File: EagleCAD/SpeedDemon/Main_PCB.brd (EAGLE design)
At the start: 77 x 46.5 mm, 77 parts, among them Q1 DMC2700, Q2 BSS138L, U2 NC7S08M, U3 LM3676, U4 STM32F072-LQFP48, X1 32.768kHz

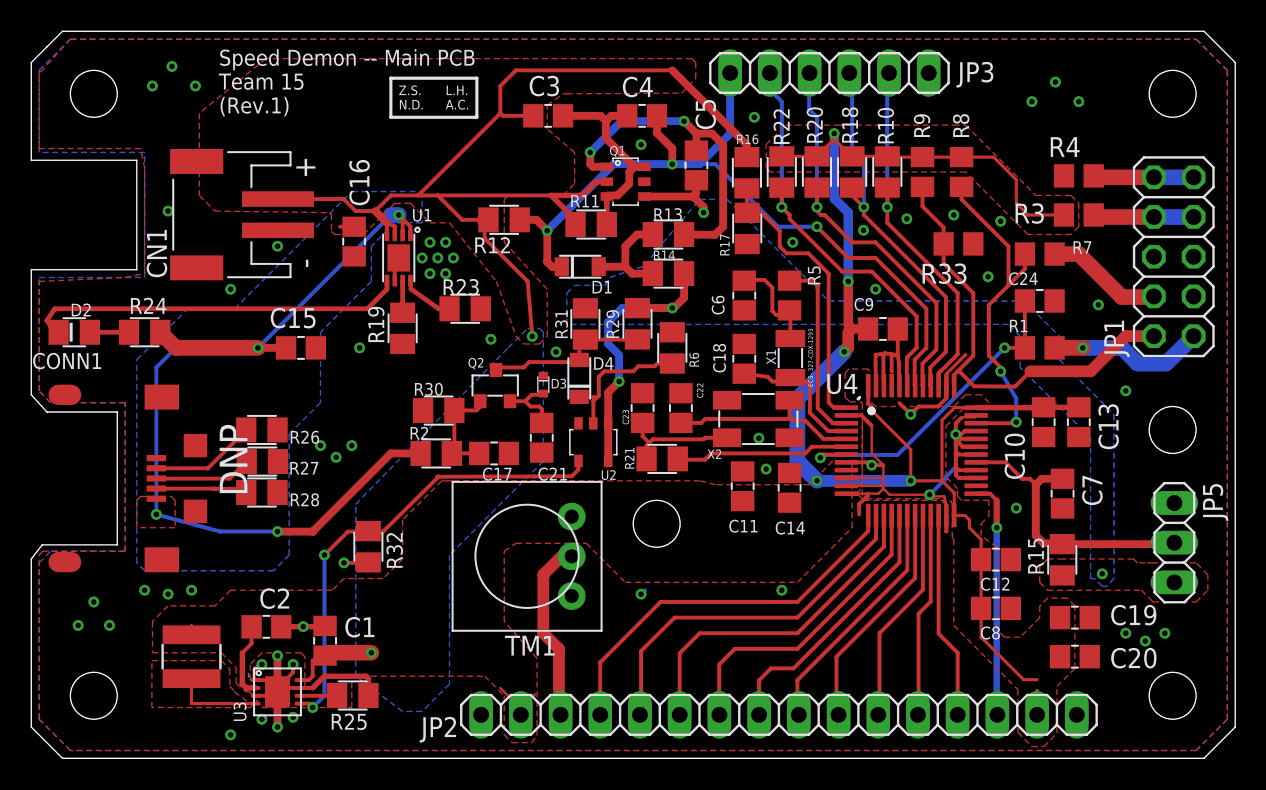
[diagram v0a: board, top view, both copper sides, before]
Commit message: final board
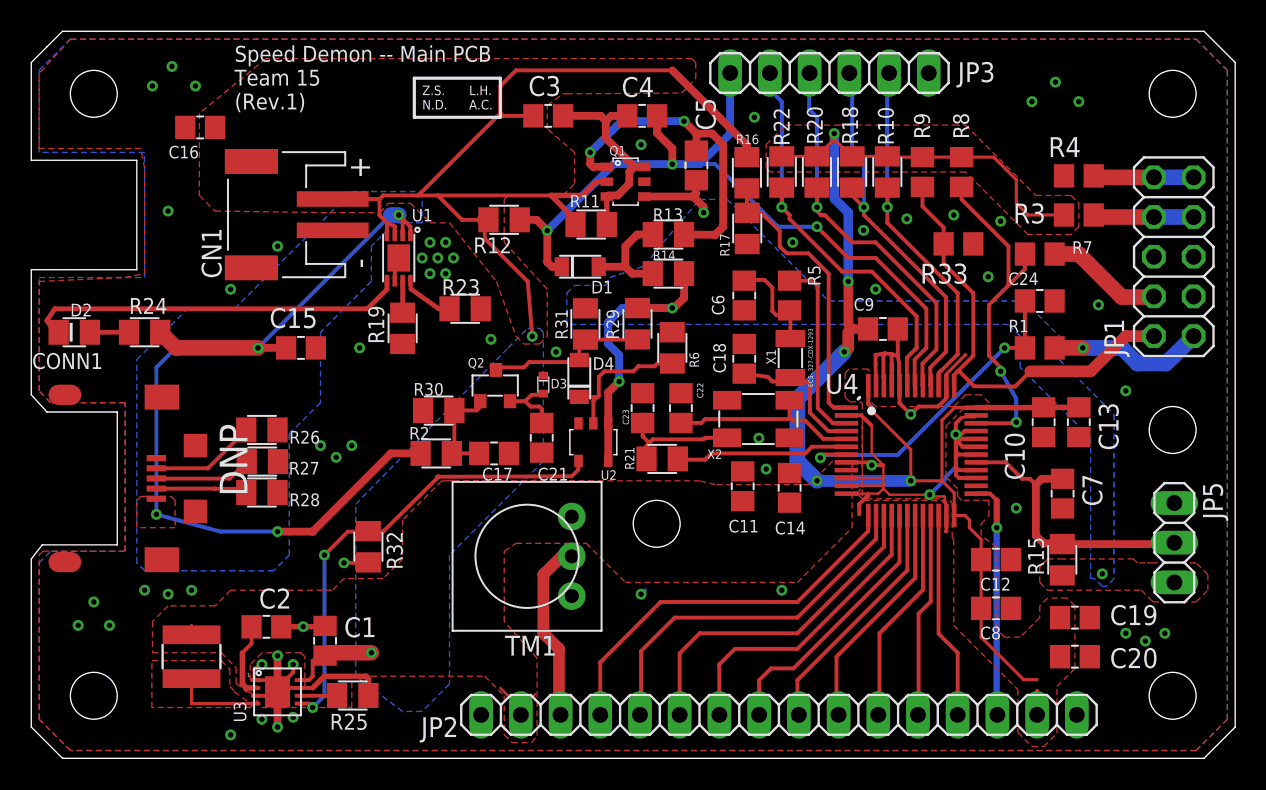
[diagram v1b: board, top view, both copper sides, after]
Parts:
- moved C16 12.3 mm to (10.8, 40.4), turned to 180 degrees
- moved CN1 3.50 mm to (15.6, 34.8)
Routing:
- net VBATT+: track 77.2 -> 72.8 mm
- net GND: track 82.9 -> 85.5 mm
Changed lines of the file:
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@@
 <setting verticaltext="up"/>
 </settings>
-<grid distance="1" unitdist="mm" unit="mm" style="lines" multiple="1" display="no" altdistance="0.05" altunitdist="mm" altunit="mm"/>
+<grid distance="0.25" unitdist="mm" unit="mm" style="lines" multiple="1" display="no" altdistance="0.05" altunitdist="mm" altunit="mm"/>
 <layers>
 <layer number="1" name="Top" color="4" fill="1" visible="yes" active="yes"/>
@@
 <dimension x1="78" y1="46.5" x2="78" y2="42.5" x3="78.5" y3="44.5" textsize="1.778" layer="51"/>
 <dimension x1="77" y1="0" x2="77" y2="21" x3="80" y3="10.5" textsize="1.778" layer="51"/>
-<text x="12" y="41.25" size="1.016" layer="21">Speed Demon -- Main PCB
+<text x="13" y="41.5" size="1.016" layer="21">Speed Demon -- Main PCB
 Team 15
 (Rev.1)</text>
-<text x="23.5" y="41.5" size="0.6096" layer="21">Z.S.
+<text x="25" y="41.5" size="0.6096" layer="21">Z.S.
 N.D.</text>
-<text x="26.5" y="41.5" size="0.6096" layer="21">L.H.
+<text x="28" y="41.5" size="0.6096" layer="21">L.H.
 A.C.</text>
-<wire x1="23" y1="43.5" x2="28.5" y2="43.5" width="0.2" layer="21"/>
-<wire x1="28.5" y1="43.5" x2="28.5" y2="41" width="0.2" layer="21"/>
-<wire x1="28.5" y1="41" x2="23" y2="41" width="0.2" layer="21"/>
-<wire x1="23" y1="41" x2="23" y2="43.5" width="0.2" layer="21"/>
+<wire x1="24.5" y1="43.5" x2="30" y2="43.5" width="0.2" layer="21"/>
+<wire x1="30" y1="43.5" x2="30" y2="41" width="0.2" layer="21"/>
+<wire x1="30" y1="41" x2="24.5" y2="41" width="0.2" layer="21"/>
+<wire x1="24.5" y1="41" x2="24.5" y2="43.5" width="0.2" layer="21"/>
 </plain>
 <attributes>
@@
 <attribute name="VALUE" x="15.98" y="23.71" size="1.27" layer="27"/>
 </element>
-<element name="C16" library="0805_generics" package="C_0805" value="4.7uF" x="20.65" y="33.05" smashed="yes" rot="R270">
-<attribute name="NAME" x="21.63" y="35.28" size="1.27" layer="25" rot="R90"/>
-<attribute name="VALUE" x="18.11" y="34.32" size="1.27" layer="27" rot="R270"/>
+<element name="C16" library="0805_generics" package="C_0805" value="4.7uF" x="10.8" y="40.35" smashed="yes" rot="R180">
+<attribute name="NAME" x="8.78" y="38.37" size="0.8" layer="25"/>
+<attribute name="VALUE" x="12.07" y="42.89" size="1.27" layer="27" rot="R180"/>
 </element>
 <element name="C18" library="LCRD_SMD_generics" package="C_0805" value="22pF" x="45.6" y="25.55" smashed="yes" rot="R270">
@@
 <attribute name="VALUE" x="53.2" y="24.92" size="1.27" layer="27"/>
 </element>
-<element name="CN1" library="adafruit" library_urn="urn:adsk.eagle:library:420" package="JST-PH-2-SMT-RA" value="" x="12.08" y="34.77" smashed="yes" rot="R90">
-<attribute name="NAME" x="8.67" y="30.68" size="1.27" layer="25" font="vector" rot="R90"/>
-<attribute name="VALUE" x="19.7" y="32.23" size="1.27" layer="27" font="vector" rot="R90"/>
+<element name="CN1" library="adafruit" library_urn="urn:adsk.eagle:library:420" package="JST-PH-2-SMT-RA" value="" x="15.58" y="34.77" smashed="yes" rot="R90">
+<attribute name="NAME" x="12.17" y="30.68" size="1.27" layer="25" font="vector" rot="R90"/>
+<attribute name="VALUE" x="23.2" y="32.23" size="1.27" layer="27" font="vector" rot="R90"/>
 </element>
 <element name="D1" library="LCRD_SMD_generics" package="D_SOD_123" value="1N4148_SOD_123" x="35.11" y="31.44" smashed="yes" rot="R180">
@@
 <wire x1="54.5" y1="24.36" x2="54.5" y2="25.75" width="0.25" layer="1"/>
 <wire x1="54.5" y1="25.75" x2="54.6" y2="25.9" width="0.25" layer="1"/>
-<wire x1="55.03" y1="24.72" x2="55.0263" y2="25.857084375" width="0.25" layer="1"/>
+<wire x1="55.03" y1="24.72" x2="55.028275" y2="25.250090625" width="0.25" layer="1"/>
+<wire x1="55.028275" y1="25.250090625" x2="55.0263" y2="25.857084375" width="0.25" layer="1"/>
 <wire x1="55.53" y1="24.47" x2="55.5" y2="24.5" width="0.25" layer="1"/>
 <wire x1="55.5" y1="24.5" x2="55.5" y2="25.28365" width="0.25" layer="1"/>
@@
 <wire x1="52.134565625" y1="21.934565625" x2="52.13" y2="21.93" width="0.25" layer="1"/>
 <contactref element="R33" pad="1"/>
+<wire x1="55.028275" y1="25.250090625" x2="55.028275" y2="23.831725" width="0.25" layer="1"/>
+<wire x1="55.028275" y1="23.831725" x2="55.03" y2="23.83" width="0.25" layer="1"/>
+<wire x1="55.53" y1="22.72" x2="55.53" y2="23.83" width="0.25" layer="1"/>
 </signal>
 <signal name="N$10">
@@
 <contactref element="R11" pad="2"/>
 <contactref element="R16" pad="2"/>
-<wire x1="20.75" y1="35" x2="22" y2="35" width="0.25" layer="1"/>
-<wire x1="22" y1="35" x2="22.75" y2="34.25" width="0.5" layer="1"/>
 <wire x1="22.75" y1="34.25" x2="22.75" y2="33.45" width="0.25" layer="1"/>
 <wire x1="22.75" y1="34.25" x2="23.246984375" y2="34.013325" width="0.25" layer="1"/>
-<wire x1="20.65" y1="34" x2="19.75" y2="34" width="0.25" layer="1"/>
-<wire x1="22" y1="35" x2="23" y2="36" width="0.25" layer="1"/>
 <wire x1="29" y1="34.44" x2="27.56" y2="34.44" width="0.25" layer="1"/>
 <wire x1="29" y1="34.44" x2="29.24" y2="34.44" width="1" layer="1"/>
-<wire x1="26" y1="36" x2="24.75" y2="36" width="0.25" layer="1"/>
-<wire x1="24.75" y1="36" x2="23" y2="36" width="0.25" layer="1"/>
+<wire x1="24.75" y1="36" x2="26" y2="36" width="0.25" layer="1"/>
 <wire x1="26" y1="36" x2="27.56" y2="34.44" width="0.25" layer="1"/>
 <wire x1="26" y1="36" x2="33.25" y2="36" width="0.25" layer="1"/>
@@
 <vertex x="11.75" y="35"/>
 <vertex x="19.1" y="34.9"/>
-<vertex x="19.2" y="34.8"/>
-<vertex x="19.2" y="33.7"/>
-<vertex x="19.4" y="33.5"/>
-<vertex x="21.25" y="33.5"/>
-<vertex x="23.25" y="35.5"/>
+<vertex x="22.3" y="34.9"/>
+<vertex x="22.85" y="35.5"/>
 <vertex x="24.25" y="35.5"/>
 <vertex x="25.5" y="34.25"/>
@@
 <wire x1="45.75" y1="39.25" x2="45.75" y2="39.07" width="0.5" layer="1"/>
 <wire x1="45.75" y1="39.07" x2="45.77" y2="38.45" width="0.5" layer="1"/>
-<wire x1="19.98" y1="35.77" x2="20.75" y2="35" width="0.25" layer="1"/>
-<wire x1="15.78" y1="35.77" x2="19.98" y2="35.77" width="0.25" layer="1"/>
+<wire x1="19.28" y1="35.77" x2="22.27" y2="35.77" width="0.25" layer="1"/>
+<wire x1="22.27" y1="35.77" x2="22.5" y2="36" width="0.25" layer="1"/>
+<wire x1="22.5" y1="36" x2="24.75" y2="36" width="0.25" layer="1"/>
+<wire x1="22.27" y1="35.77" x2="22.27" y2="34.73" width="0.25" layer="1"/>
+<wire x1="22.27" y1="34.73" x2="22.75" y2="34.25" width="0.25" layer="1"/>
 </signal>
 <signal name="OSC32_OUT">
